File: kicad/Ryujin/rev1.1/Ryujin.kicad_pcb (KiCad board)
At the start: 2 copper layers, 56 x 77 mm, 26 parts, among them J1 Screw_Terminal_01x06, J3 Conn_01x14_Socket, J4 Conn_01x14_Socket, Q1 IRLML6244, U1 74LVC1G17, U2 R-78E5.0-0.5, U3 W25Q32JVSS, U4 SHTC3, U5 74AHCT1G125, U6 TMUX1119DBVR

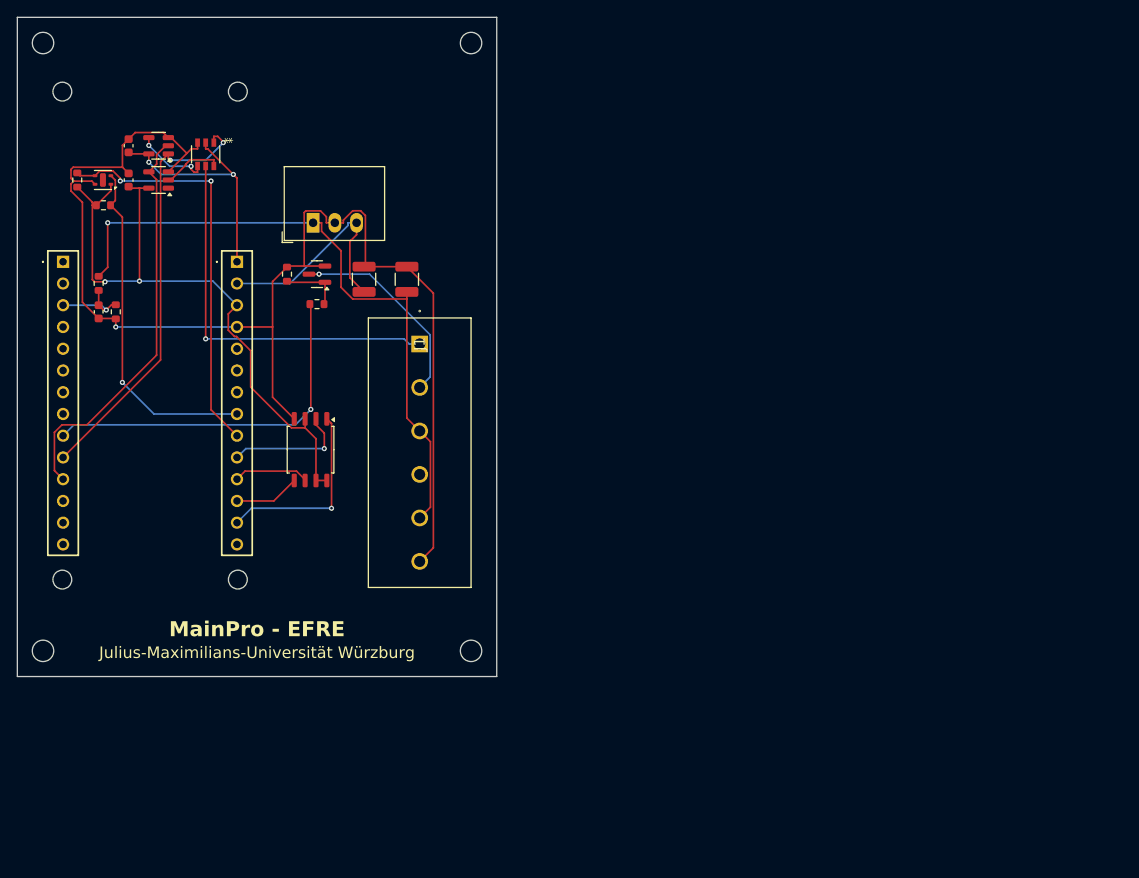
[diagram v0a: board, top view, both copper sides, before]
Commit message: Highway to Hades
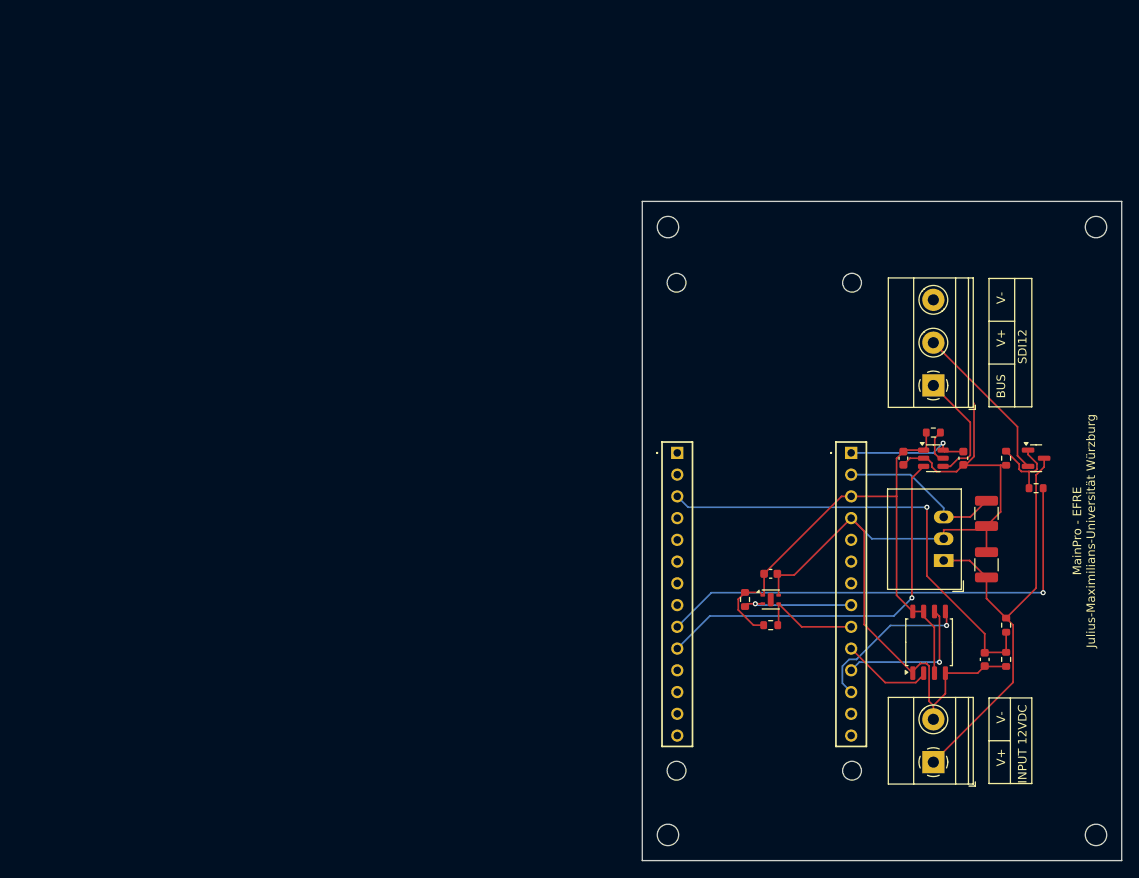
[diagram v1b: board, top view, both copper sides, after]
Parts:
- removed U5: 74AHCT1G125, Package_TO_SOT_SMD:SOT-23-5
- removed U6: TMUX1119DBVR, footprints:DBV0006A
- added C5: 0.1uF, Capacitor_SMD:C_0603_1608Metric, F.Cu at (232.5, 70.5)
- added J2: SDI12, TerminalBlock_Phoenix:TerminalBlock_Phoenix_MKDS-1,5-3_1x03_P5.00mm_Horizontal, F.Cu at (236.0, 62.0)
- added R1: 47k, Resistor_SMD:R_0603_1608Metric, F.Cu at (236.0, 67.5)
- J1: value Screw_Terminal_01x06 -> BAT; footprint ThirdParty:SMKDSN-1-5-6-5-08_3D -> TerminalBlock_Phoenix:TerminalBlock_Phoenix_MKDS-1,5-2_1x02_P5.00mm_Horizontal
- U1: value 74LVC1G17 -> TXS0101DBV; footprint Package_TO_SOT_SMD:SOT-23-5 -> Package_TO_SOT_SMD:SOT-23-6
- moved R5 113.3 mm to (244.5, 90.0)
- moved R4 111.6 mm to (244.5, 94.0)
- moved C3 111.2 mm to (242.0, 94.0)
- moved C4 104.1 mm to (239.5, 70.5)
- moved R7 96.3 mm to (217.0, 90.0), turned to 180 degrees
- moved U1 96.2 mm to (236.0, 70.5), turned to 0 degrees
- moved U4 92.1 mm to (217.0, 87.0), turned to 0 degrees
- moved C6 88.0 mm to (217.0, 84.0), turned to 0 degrees
- moved R6 88.0 mm to (214.0, 87.0), turned to 90 degrees
- moved Q1 86.7 mm to (248.0, 70.5), turned to 0 degrees
- moved R2 86.7 mm to (248.0, 74.0), turned to 0 degrees
- moved R3 86.7 mm to (244.5, 70.5), turned to 90 degrees
- moved U2 83.6 mm to (237.2, 82.4), turned to 90 degrees
- moved C2 77.7 mm to (242.2, 76.9), turned to -90 degrees
- moved J1 77.4 mm to (236.0, 106.0), turned to 90 degrees
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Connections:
- C4 pad 1: /5V -> /GND
- C4 pad 2: /GND -> /5V
- J1 pad 1: /BUS -> /BAT+
- J1 pad 2: /SDI- -> /GND
- J3 pad 11: /D2 -> unconnected-(J3-~D2-Pad11)
- J4 pad 13: /D7 -> unconnected-(J4-~D7-Pad13)
- J4 pad 5: /RTS -> unconnected-(J4-RESET-Pad5)
- Q1 pad 2: /GND -> /SDI+
- Q1 pad 3: /SDI- -> /BAT+
- U1 pad 1: unconnected-(U1-NC-Pad1) -> /3V3
- U1 pad 2: Net-(U6-S2) -> /GND
- U1 pad 3: /GND -> /D1
- U1 pad 4: /D2 -> /BUS
- U1 pad 5: /3V3 -> Net-(U1-OE)
- U3 pad 1: /D7 -> /GND
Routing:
- net /GND: track 153.8 -> 106.1 mm, vias 1 -> 0
- net /D2: track 47.5 -> 0.00 mm
- net /A1: track 9.49 -> 54.4 mm
- net /SDA: track 47.7 -> 12.1 mm, vias 2 -> 0
- net /BUS: track 45.4 -> 13.7 mm, vias 1 -> 0
- net /SCL: track 40.1 -> 13.5 mm
- net /SDI-: track 23.7 -> 0.00 mm, vias 1 -> 0
- net /BAT+: track 76.5 -> 53.0 mm, vias 1 -> 0
- net /D7: track 22.4 -> 0.00 mm, vias 1 -> 0
- net /SDI+: track 0.00 -> 19.0 mm
- net /5V: track 29.4 -> 14.5 mm, vias 2 -> 1
- net /D0: track 42.6 -> 56.6 mm
- net /3V3: track 75.2 -> 63.5 mm, vias 2 -> 0
- net /COPI: track 7.68 -> 19.3 mm, vias 0 -> 1
- net Net-(U6-S1): track 8.83 -> 0.00 mm, vias 2 -> 0
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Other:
- board text added: "BUS"
- board text added: "INPUT 12VDC"
- board text added: "MainPro - EFRE Julius-Maximilians-Universität Würzburg"
- board text added: "SDI12"
- board text added: "V+"
- board text added: "V-"
- board text removed: "Julius-Maximilians-Universität Würzburg"
- board text removed: "MainPro - EFRE"
